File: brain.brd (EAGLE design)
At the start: 100 x 80.3 mm, 28 parts, among them IC1 LP2950ACZ-3.3, IC2 LP2950ACZ-3.3, U1 TINY45-20-DIP, U4 TINY45-20-DIP, U5 TINY45-20-DIP, U6 TINY45-20-DIP

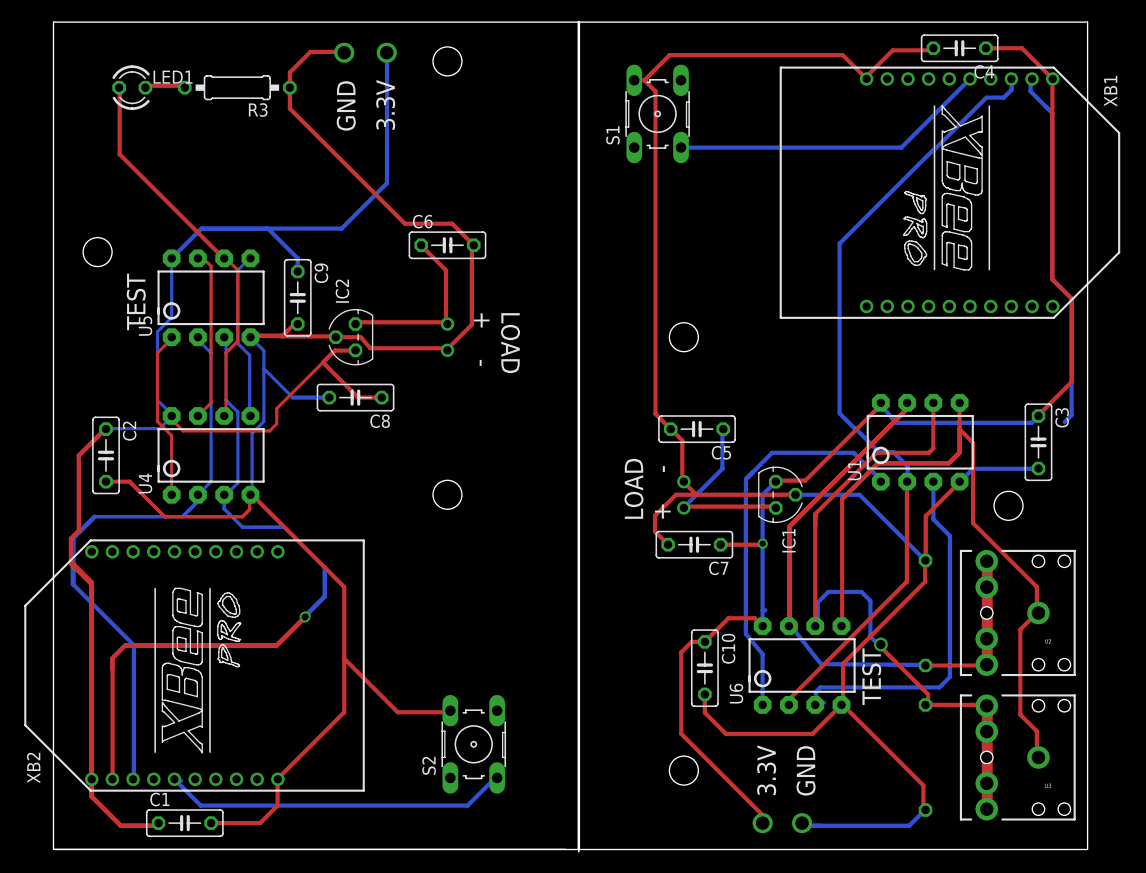
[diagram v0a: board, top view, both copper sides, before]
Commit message: Most recent board changes. also, added the arduino files for the attiny.
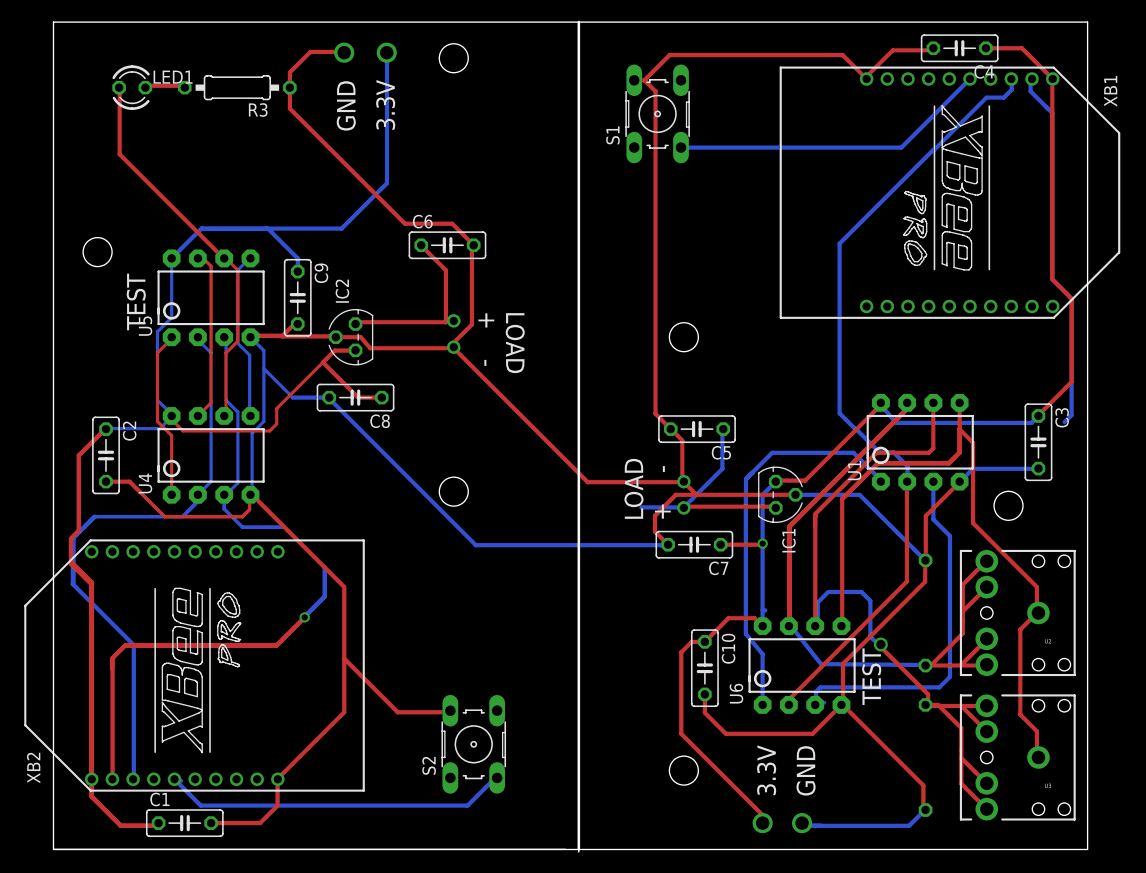
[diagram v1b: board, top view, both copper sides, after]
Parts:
- moved U$6 0.68 mm to (40.0, 34.6)
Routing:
- net N$45: track 0.00 -> 38.9 mm
- net N$43: track 0.00 -> 27.7 mm
- net N$42: track 0.00 -> 15.7 mm
- net N$40: track 0.00 -> 9.24 mm
- net N$44: track 0.00 -> 3.96 mm
- net N$41: track 0.00 -> 3.45 mm
- net PB11: track 26.5 -> 27.6 mm
- net VIN2: track 17.5 -> 18.1 mm
- net N$31: vias 1 -> 0
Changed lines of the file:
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@@
 <text x="59.69" y="31.75" size="1.778" layer="21" rot="R90">LOAD
 +    -</text>
-<text x="40.64" y="52.07" size="1.778" layer="21" rot="SR270">LOAD
+<text x="41.0972" y="52.07" size="1.778" layer="21" rot="SR270">LOAD
 +    -</text>
 <text x="80.01" y="13.97" size="1.778" layer="21" rot="R90">TEST</text>
@@
 <text x="31.231890625" y="74.41405" size="1.778" layer="21" rot="R270">3.3V</text>
 <text x="27.421890625" y="74.41405" size="1.778" layer="21" rot="R270">GND</text>
-<rectangle x1="89.7636" y1="17.526" x2="90.8304" y2="28.194" layer="1"/>
-<rectangle x1="89.7636" y1="3.5052" x2="90.8304" y2="14.1732" layer="1"/>
 <hole x="4.2672" y="57.7596" drill="2.8"/>
 <hole x="92.3544" y="33.2232" drill="2.8"/>
 <text x="48.006" y="68.8848" size="2.54" layer="22" rot="MR270">Water Management System</text>
 <text x="97.536" y="65.2272" size="2.54" layer="22" rot="MR270">Water Management System</text>
+<dimension x1="0" y1="0" x2="100" y2="0" x3="50" y3="-2.286" textsize="1.778" layer="16" unit="inch"/>
+<dimension x1="100" y1="-0.01" x2="100" y2="80" x3="109.2708" y3="39.995" textsize="1.778" layer="16" unit="inch"/>
 </plain>
 <attributes>
@@
 <attribute name="OC_FARNELL" value="176432" x="-21.59" y="-36.83" size="1.778" layer="27" rot="R90" display="off"/>
 </element>
-<element name="U$6" library="seniordesign" package="SUNNYBUDDYMOUNT" value="SUNNYBUDDYMOUNT" x="39.37" y="34.29" rot="R180"/>
+<element name="U$6" library="seniordesign" package="SUNNYBUDDYMOUNT" value="SUNNYBUDDYMOUNT" x="39.9796" y="34.5948" rot="R180"/>
 <element name="C1" library="rcl" package="C050-025X075" value="bypass" x="12.7" y="2.54"/>
 <element name="C2" library="rcl" package="C050-025X075" value="bypass" x="5.08" y="38.1" rot="R270"/>
@@
 <wire x1="37.9476" y1="50.9778" x2="29.2608" y2="50.9778" width="0.4064" layer="1"/>
 <wire x1="29.2608" y1="50.9778" x2="29.21" y2="50.8" width="0.4064" layer="1"/>
-<wire x1="37.9476" y1="50.9778" x2="38.1" y2="50.8" width="0.4064" layer="1"/>
+<wire x1="37.9476" y1="50.9778" x2="38.7096" y2="51.1048" width="0.4064" layer="1"/>
 </signal>
 <signal name="N$8">
@@
 <wire x1="38.1762" y1="13.2588" x2="33.2994" y2="13.2588" width="0.4064" layer="1"/>
 <wire x1="33.2994" y1="13.2588" x2="28.1178" y2="18.4404" width="0.4064" layer="1"/>
-<wire x1="38.1762" y1="48.4632" x2="38.1" y2="48.26" width="0" layer="19" extent="1-1"/>
+<wire x1="38.1762" y1="48.4632" x2="38.7096" y2="48.5648" width="0" layer="19" extent="1-1"/>
 <wire x1="37.9476" y1="48.4632" x2="38.1762" y2="48.4632" width="0" layer="19" extent="1-1"/>
 </signal>
@@
 <wire x1="73.681209375" y1="32.28335" x2="85.09" y2="43.18" width="0" layer="19" extent="1-1"/>
 <wire x1="84.328" y1="13.97" x2="73.66848125" y2="21.63234375" width="0" layer="19" extent="1-1"/>
-<wire x1="84.328" y1="13.97" x2="89.9668" y2="13.97" width="0.4064" layer="1"/>
-<wire x1="89.9668" y1="13.97" x2="90.2208" y2="13.716" width="0.4064" layer="1"/>
-<wire x1="90.2208" y1="13.716" x2="90.2208" y2="3.9192" width="0.4064" layer="1"/>
-<wire x1="90.2208" y1="3.9192" x2="90.25" y2="3.89" width="0.4064" layer="1"/>
+<wire x1="84.328" y1="13.97" x2="85.5472" y2="13.97" width="0.4064" layer="1"/>
+<wire x1="85.5472" y1="13.97" x2="87.7824" y2="11.7348" width="0.4064" layer="1"/>
+<wire x1="87.7824" y1="11.7348" x2="87.7824" y2="9.6012" width="0.4064" layer="1"/>
+<wire x1="87.7824" y1="8.8392" x2="87.7824" y2="6.3576" width="0.4064" layer="1"/>
+<wire x1="87.7824" y1="6.3576" x2="90.25" y2="3.89" width="0.4064" layer="1"/>
+<wire x1="87.7824" y1="9.6012" x2="87.7824" y2="8.8392" width="0.4064" layer="1"/>
+<wire x1="87.7824" y1="8.8392" x2="90.3732" y2="6.2484" width="0.4064" layer="1"/>
 </signal>
 <signal name="PB51">
@@
 <wire x1="6.941971875" y1="19.725359375" x2="21.587840625" y2="19.725359375" width="0.4064" layer="1"/>
 <wire x1="21.587840625" y1="19.725359375" x2="24.3815625" y2="22.51908125" width="0.4064" layer="1"/>
-<via x="24.3815625" y="22.51908125" extent="1-16" drill="0.6" shape="square"/>
 </signal>
 <signal name="N$32">
@@
 <wire x1="94.488" y1="73.3044" x2="96.1644" y2="71.628" width="0.4064" layer="16"/>
 </signal>
+<signal name="N$40">
+<wire x1="84.4296" y1="13.8684" x2="86.868" y2="13.8684" width="0.4064" layer="1"/>
+<wire x1="87.7824" y1="13.8684" x2="90.2208" y2="13.8684" width="0.4064" layer="1"/>
+<wire x1="86.868" y1="13.8684" x2="87.7824" y2="13.8684" width="0.4064" layer="1"/>
+<wire x1="87.7824" y1="13.8684" x2="90.2208" y2="11.43" width="0.4064" layer="1"/>
+</signal>
+<signal name="N$41">
+<wire x1="87.7824" y1="17.8308" x2="90.2208" y2="20.2692" width="0.4064" layer="1"/>
+</signal>
+<signal name="N$42">
+<wire x1="84.582" y1="17.6784" x2="84.7344" y2="17.6784" width="0.4064" layer="1"/>
+<wire x1="84.7344" y1="17.6784" x2="87.9348" y2="20.8788" width="0.4064" layer="1"/>
+<wire x1="87.9348" y1="20.8788" x2="87.9348" y2="22.098" width="0.4064" layer="1"/>
+<wire x1="87.9348" y1="23.0124" x2="87.9348" y2="25.6032" width="0.4064" layer="1"/>
+<wire x1="87.9348" y1="25.6032" x2="90.0684" y2="27.7368" width="0.4064" layer="1"/>
+<wire x1="87.9348" y1="22.098" x2="87.9348" y2="23.0124" width="0.4064" layer="1"/>
+<wire x1="87.9348" y1="23.0124" x2="90.2208" y2="25.2984" width="0.4064" layer="1"/>
+</signal>
+<signal name="N$43">
+<wire x1="38.862" y1="48.3108" x2="51.6636" y2="35.5092" width="0.4064" layer="1"/>
+<wire x1="51.6636" y1="35.5092" x2="61.2648" y2="35.5092" width="0.4064" layer="1"/>
+</signal>
+<signal name="N$44">
+<wire x1="56.8452" y1="33.0708" x2="60.8076" y2="33.0708" width="0.4064" layer="16"/>
+</signal>
+<signal name="N$45">
+<wire x1="26.5176" y1="43.7388" x2="40.8432" y2="29.4132" width="0.4064" layer="16"/>
+<wire x1="40.8432" y1="29.4132" x2="59.436" y2="29.4132" width="0.4064" layer="16"/>
+</signal>
 </signals>
